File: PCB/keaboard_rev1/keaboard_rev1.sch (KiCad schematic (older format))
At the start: 55 parts, among them K01 KEYSW, K02 KEYSW, K03 KEYSW, K04 KEYSW, K05 KEYSW, K06 KEYSW, K07 KEYSW, K08 KEYSW, K09 KEYSW, K10 KEYSW, K11 KEYSW, K12 KEYSW, K13 KEYSW, K14 KEYSW, K15 KEYSW, K16 KEYSW, K17 KEYSW, K18 KEYSW, K19 KEYSW, K20 KEYSW, K21 KEYSW, K22 KEYSW, K23 KEYSW, K24 KEYSW, K25 KEYSW, U1 ProMicro

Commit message: Update pcb image, generate gerber
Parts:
- BAT1: footprint parts:DF3A-3P-2DS -> parts:DF3A-3P-2DS_reversible
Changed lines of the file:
@@
 F 0 "BAT1" V 4642 6800 50  0000 R CNN
 F 1 "Battery" H 4642 6845 50  0001 R CNN
-F 2 "parts:DF3A-3P-2DS" V 4750 6860 50  0001 C CNN
+F 2 "parts:DF3A-3P-2DS_reversible" V 4750 6860 50  0001 C CNN
 F 3 "~" V 4750 6860 50  0001 C CNN
 	1    4750 6800

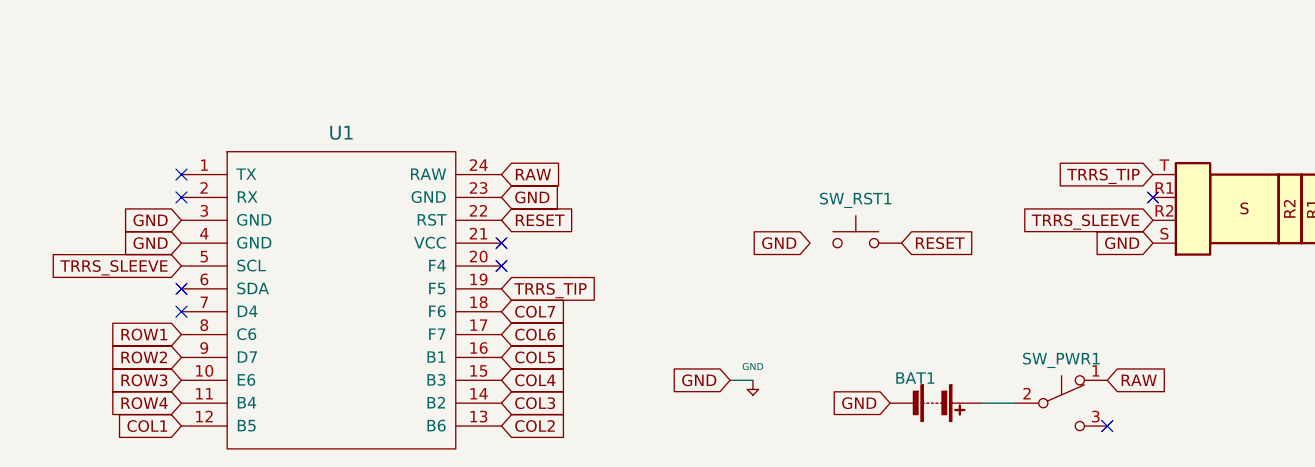
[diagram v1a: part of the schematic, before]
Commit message: Update schematic, update footprints, start updating layout
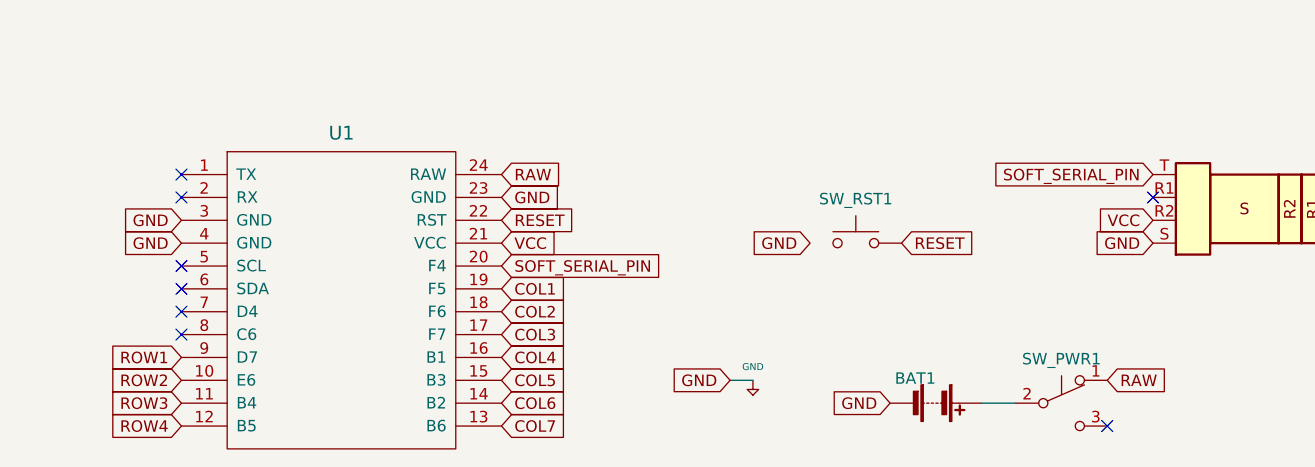
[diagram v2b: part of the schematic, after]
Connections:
- net COL1: now also U1.19 (F5); no longer U1.12 (B5)
- net COL2: now also U1.18 (F6); no longer U1.13 (B6)
- net COL3: now also U1.17 (F7); no longer U1.14 (B2)
- net COL4: now also U1.16 (B1); no longer U1.15 (B3)
- net COL5: now also U1.15 (B3); no longer U1.16 (B1)
- net COL6: now also U1.14 (B2); no longer U1.17 (F7)
- net COL7: now also U1.13 (B6); no longer U1.18 (F6)
- net ROW1: now also U1.9 (D7); no longer U1.8 (C6)
- net ROW2: now also U1.10 (E6); no longer U1.9 (D7)
- net ROW3: now also U1.11 (B4); no longer U1.10 (E6)
- net ROW4: now also U1.12 (B5); no longer U1.11 (B4)
- net SOFT_SERIAL_PIN: now reaches U1.20 (F4)
- net SOFT_SERIAL_PIN: now also TRRS1.T
- net VCC: now reaches U1.21 (VCC)
- net VCC: now also TRRS1.R2
- net TRRS_SLEEVE: no longer names the net of U1.5 (SCL)
- net TRRS_SLEEVE: no longer TRRS1.R2
- removed net TRRS_TIP: TRRS1.T, U1.19 (F5)
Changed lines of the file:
@@
 	1    0    0    -1
 $EndComp
+Text GLabel 2850 6900 2    50   Input ~ 0
+COL7
+Text GLabel 2850 6300 2    50   Input ~ 0
+COL1
 Text GLabel 2850 6400 2    50   Input ~ 0
-COL7
+COL2
+Text GLabel 2850 6500 2    50   Input ~ 0
+COL3
+Text GLabel 2850 6600 2    50   Input ~ 0
+COL4
+Text GLabel 2850 6700 2    50   Input ~ 0
+COL5
+Text GLabel 2850 6800 2    50   Input ~ 0
+COL6
+Text GLabel 1450 6800 0    50   Input ~ 0
+ROW3
+Text GLabel 1450 6700 0    50   Input ~ 0
+ROW2
+Text GLabel 1450 6600 0    50   Input ~ 0
+ROW1
 Text GLabel 1450 6900 0    50   Input ~ 0
-COL1
-Text GLabel 2850 6900 2    50   Input ~ 0
-COL2
-Text GLabel 2850 6800 2    50   Input ~ 0
-COL3
-Text GLabel 2850 6700 2    50   Input ~ 0
-COL4
-Text GLabel 2850 6600 2    50   Input ~ 0
-COL5
-Text GLabel 2850 6500 2    50   Input ~ 0
-COL6
-Text GLabel 1450 6700 0    50   Input ~ 0
-ROW3
-Text GLabel 1450 6600 0    50   Input ~ 0
-ROW2
-Text GLabel 1450 6500 0    50   Input ~ 0
-ROW1
-Text GLabel 1450 6800 0    50   Input ~ 0
 ROW4
 Wire Wire Line
@@
 NoConn ~ 1450 6300
 NoConn ~ 1450 6400
-NoConn ~ 2850 6200
-NoConn ~ 2850 6100
 Text GLabel 3850 6700 0    50   Input ~ 0
 GND
@@
 	-1   0    0    1
 $EndComp
-Text GLabel 2850 6300 2    50   Input ~ 0
-TRRS_TIP
+Text GLabel 2850 6200 2    50   Input ~ 0
+SOFT_SERIAL_PIN
 Text GLabel 5700 5800 0    50   Input ~ 0
-TRRS_TIP
+SOFT_SERIAL_PIN
 Text GLabel 5700 6000 0    50   Input ~ 0
-TRRS_SLEEVE
-Text GLabel 1450 6200 0    50   Input ~ 0
-TRRS_SLEEVE
+VCC
+Text GLabel 2850 6100 2    50   Input ~ 0
+VCC
 NoConn ~ 5700 5900
 Text GLabel 5700 6100 0    50   Input ~ 0
@@
 	0    1    1    0
 $EndComp
+NoConn ~ 1450 6200
+NoConn ~ 1450 6500
 $EndSCHEMATC
